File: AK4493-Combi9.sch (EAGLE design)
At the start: 199 parts, among them IC1 LT3042, IC10 LT3042, IC2 LT3042, IC3 LM317MQDCYR, IC4 LM317MQDCYR, IC5 LT3042, IC6 LT3042, IC8 LT3042, J1 XR2A-0811-N, J10 XR2A-0811-N, J12 XR2A-0811-N, J17 XR2A-0811-N, J3 SJ-63033A, J4 1935255, J5 XR2A-0811-N, J6 1935255, J7 1935200, J8 XR2A-0811-N, J9 1935200, U1 LM317MTG, U2 LM317MTG

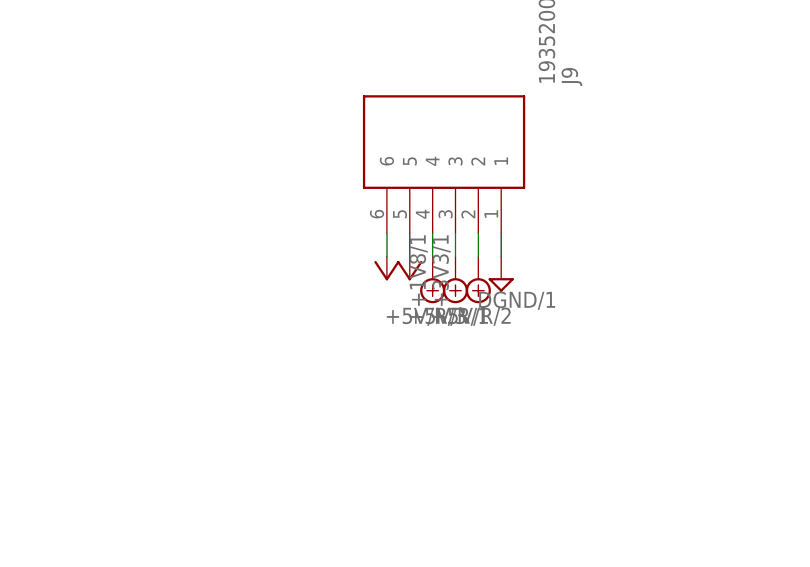
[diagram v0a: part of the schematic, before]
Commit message: Progress
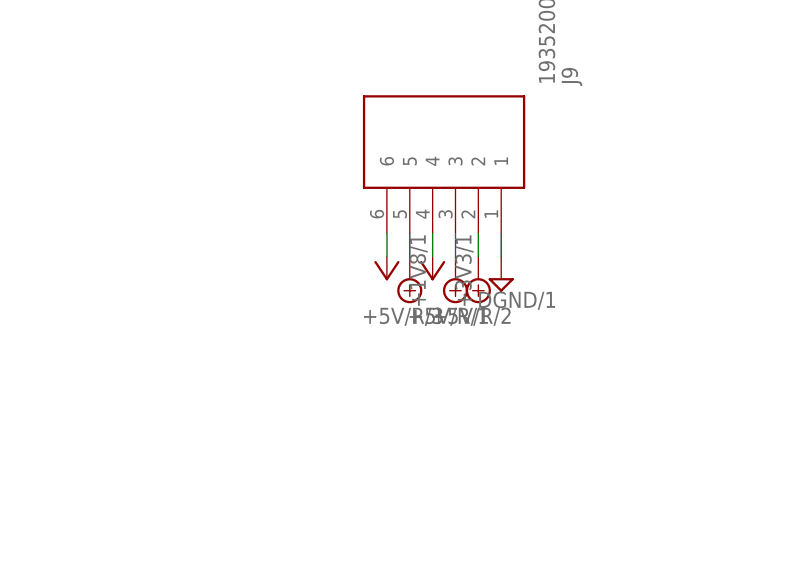
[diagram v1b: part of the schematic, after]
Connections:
- net +3V3/1: now also J9.4; no longer J9.5
- net +5V/R/3: now also J9.5; no longer J9.4
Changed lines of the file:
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@@
 <attribute name="VALUE" x="-326.39" y="167.005" size="1.778" layer="96" rot="R180"/>
 </instance>
-<instance part="SUPPLY19" gate="G$1" x="-332.74" y="170.18" smashed="yes" rot="R180">
-<attribute name="VALUE" x="-328.93" y="167.005" size="1.778" layer="96" rot="R180"/>
+<instance part="SUPPLY19" gate="G$1" x="-335.28" y="170.18" smashed="yes" rot="R180">
+<attribute name="VALUE" x="-331.47" y="167.005" size="1.778" layer="96" rot="R180"/>
 </instance>
-<instance part="+3V8" gate="G$1" x="-335.28" y="170.18" smashed="yes" rot="R180">
-<attribute name="VALUE" x="-332.74" y="175.26" size="1.778" layer="96" rot="R270"/>
+<instance part="+3V8" gate="G$1" x="-332.74" y="170.18" smashed="yes" rot="R180">
+<attribute name="VALUE" x="-330.2" y="175.26" size="1.778" layer="96" rot="R270"/>
 </instance>
 <instance part="+3V9" gate="G$1" x="-337.82" y="170.18" smashed="yes" rot="R180">
@@
 </segment>
 <segment>
-<wire x1="-332.74" y1="175.26" x2="-332.74" y2="172.72" width="0.1524" layer="91"/>
 <pinref part="SUPPLY19" gate="G$1" pin="+5V/R/3"/>
-<pinref part="J9" gate="G$1" pin="4"/>
+<pinref part="J9" gate="G$1" pin="5"/>
+<wire x1="-335.28" y1="172.72" x2="-335.28" y2="175.26" width="0.1524" layer="91"/>
 </segment>
 </net>
@@
 </segment>
 <segment>
-<wire x1="-335.28" y1="172.72" x2="-335.28" y2="175.26" width="0.1524" layer="91"/>
-<pinref part="+3V8" gate="G$1" pin="+3V3/1"/>
-<pinref part="J9" gate="G$1" pin="5"/>
-</segment>
-<segment>
 <pinref part="LDO1" gate="G$1" pin="EN"/>
 <wire x1="-454.66" y1="170.18" x2="-457.2" y2="170.18" width="0.1524" layer="91"/>
@@
 <pinref part="+3V11" gate="G$1" pin="+3V3/1"/>
 </segment>
-</net>
+<segment>
+<pinref part="+3V8" gate="G$1" pin="+3V3/1"/>
+<pinref part="J9" gate="G$1" pin="4"/>
+<wire x1="-332.74" y1="172.72" x2="-332.74" y2="175.26" width="0.1524" layer="91"/>
+</segment>
+</net>
